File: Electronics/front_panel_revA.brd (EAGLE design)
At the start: 100.3 x 111.3 mm, 0 parts

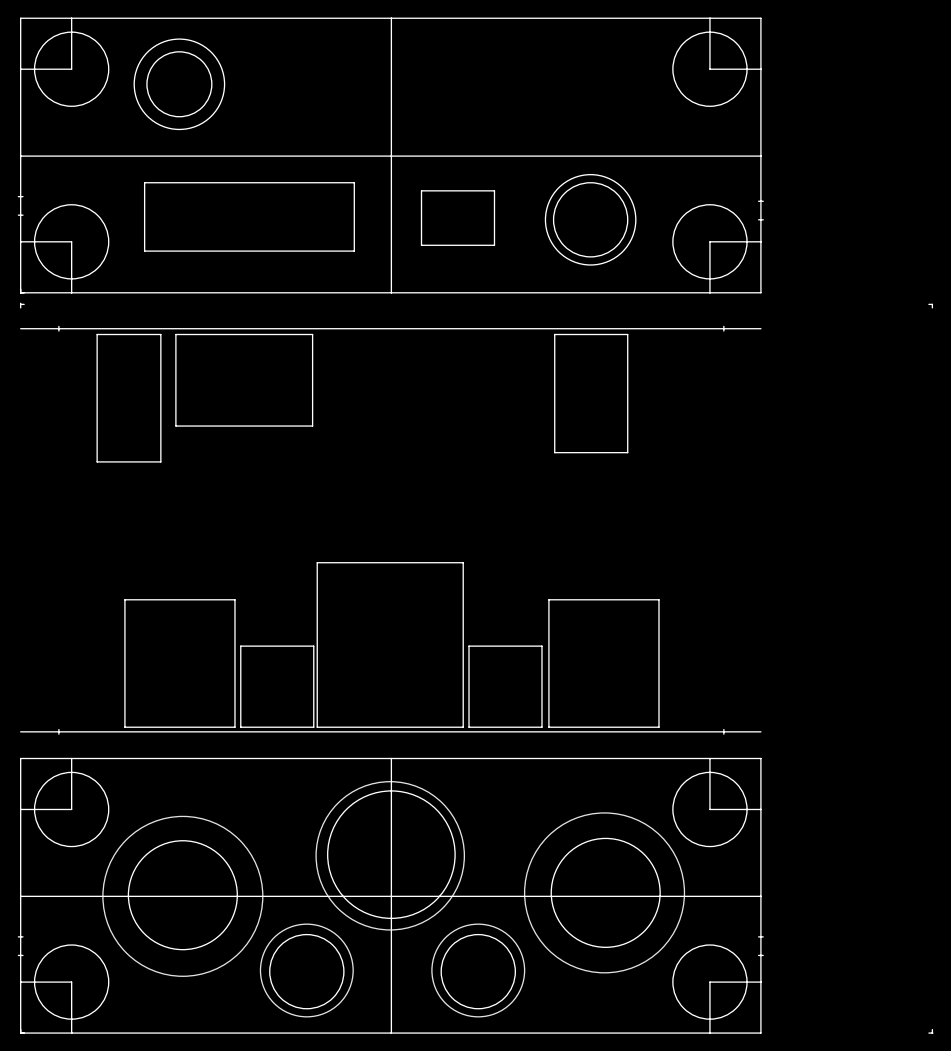
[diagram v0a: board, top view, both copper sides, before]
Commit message: Electronics: finished RevA
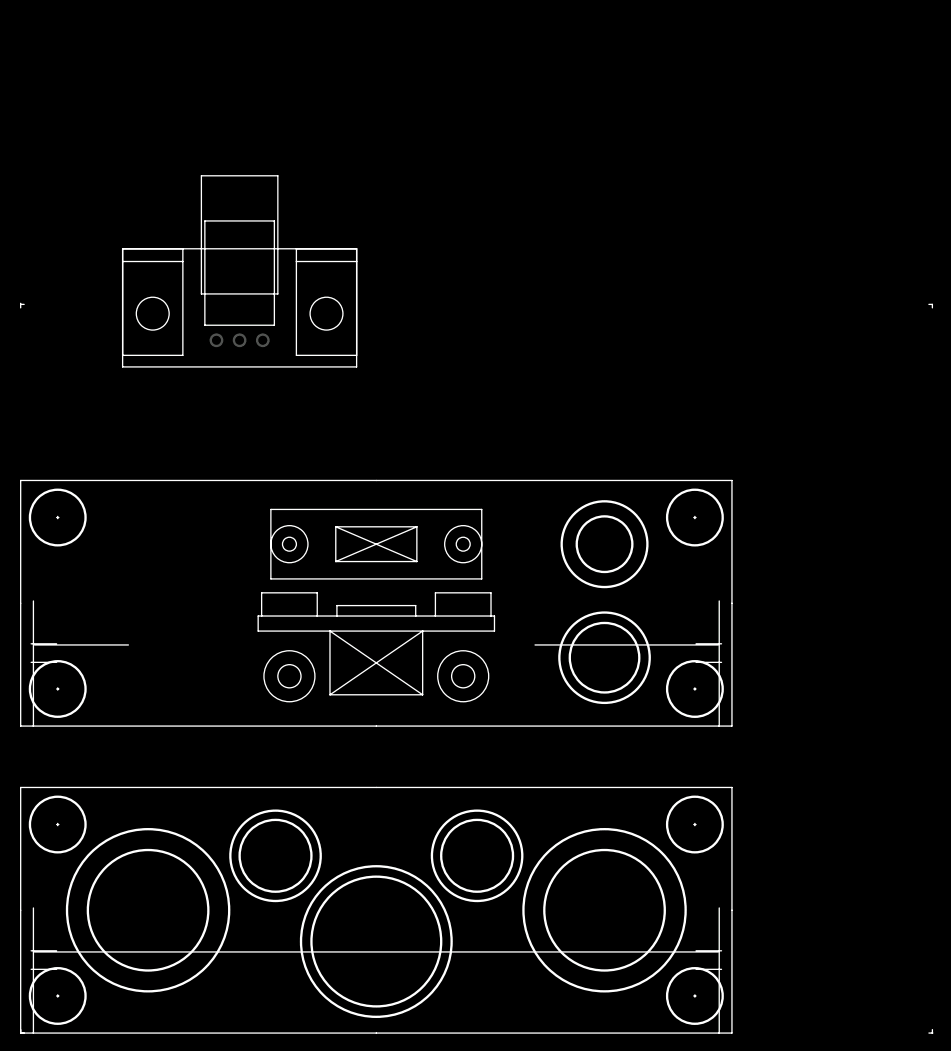
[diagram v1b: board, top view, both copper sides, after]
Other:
- board size 100.3 x 111.3 mm -> 100 x 94 mm
